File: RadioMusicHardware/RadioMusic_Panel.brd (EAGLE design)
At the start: 128.5 x 20 mm, 13 parts, among them X1 VERT_SD_CARD

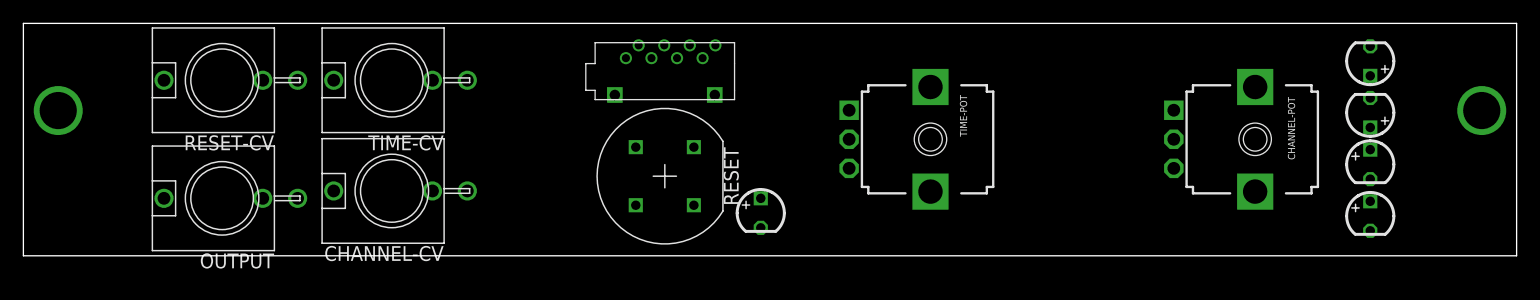
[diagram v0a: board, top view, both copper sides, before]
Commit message: Panel design
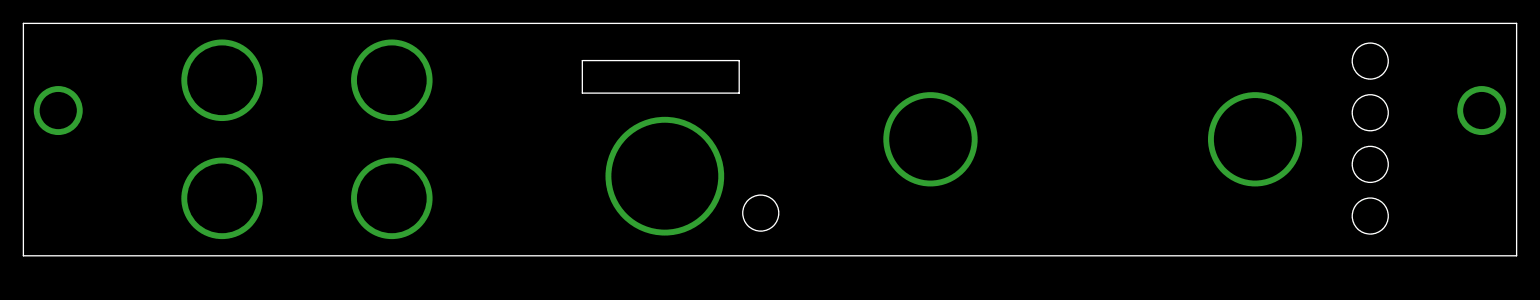
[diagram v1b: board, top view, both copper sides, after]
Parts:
- removed CHANNEL-CV, OUTPUT, RESET-CV, TIME-CV: (no value), thonkiconn:WQP-PJ301M-12_JACK
- removed CHANNEL-POT, TIME-POT: 50k, TomW:EVUF
- removed LED1, LED2, LED3, LED4, LED5: (no value), TomW:LED3MM
- removed RESET: D6_PUSH_SWITCH, TomW:D6_BUTTON_RND
- removed X1: VERT_SD_CARD, TomW:VERT_MICROSD
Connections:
- removed net +3.3V_F: TIME-POT.3
- removed net GND_F: CHANNEL-CV.P$3
- removed net LED3_F: LED3.A
- removed net LED4_F: LED4.A
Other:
- outline, holes or cut-outs redrawn
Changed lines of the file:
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@@
 <setting verticaltext="up"/>
 </settings>
-<grid distance="25" unitdist="mil" unit="mm" style="lines" multiple="1" display="yes" altdistance="8" altunitdist="mil" altunit="mil"/>
+<grid distance="25" unitdist="mil" unit="mm" style="lines" multiple="1" display="yes" altdistance="0.1" altunitdist="mm" altunit="mm"/>
 <layers>
 <layer number="1" name="Top" color="4" fill="1" visible="yes" active="yes"/>
@@
 <wire x1="128.5" y1="0" x2="128.5" y2="20" width="0.0254" layer="20"/>
 <wire x1="128.5" y1="20" x2="0" y2="20" width="0.0254" layer="20"/>
-<wire x1="130.75" y1="10" x2="-9.25" y2="10" width="0.1" layer="51"/>
-<wire x1="64.25" y1="-9.5" x2="64.25" y2="30.5" width="0.1" layer="51"/>
+<rectangle x1="48.1" y1="14" x2="61.6" y2="16.8" layer="46"/>
+<hole x="63.455" y="3.675" drill="3.1"/>
+<hole x="115.906" y="16.756" drill="3.1"/>
+<hole x="115.906" y="12.311" drill="3.1"/>
+<hole x="115.906" y="7.866" drill="3.1"/>
+<hole x="115.906" y="3.421" drill="3.1"/>
 </plain>
 <attributes>
@@
 </autorouter>
 <elements>
-<element name="CHANNEL-POT" library="TomW" package="EVUF" value="50k" x="106" y="10.025" smashed="yes" rot="R270">
-<attribute name="NAME" x="108.825" y="13.66" size="0.6096" layer="25" rot="R270"/>
-<attribute name="VALUE" x="101.58" y="11.985" size="0.6096" layer="27" rot="R270"/>
-</element>
-<element name="CHANNEL-CV" library="thonkiconn" package="WQP-PJ301M-12_JACK" value="" x="31.705" y="5.58" rot="R90"/>
-<element name="RESET-CV" library="thonkiconn" package="WQP-PJ301M-12_JACK" value="" x="17.1" y="15.105" rot="R90"/>
-<element name="OUTPUT" library="thonkiconn" package="WQP-PJ301M-12_JACK" value="" x="17.1" y="4.945" rot="R90"/>
-<element name="TIME-POT" library="TomW" package="EVUF" value="50k" x="78.06" y="10.025" smashed="yes" rot="R270">
-<attribute name="NAME" x="80.6" y="13.835" size="0.6096" layer="25" rot="R270"/>
-<attribute name="VALUE" x="74.25" y="13.835" size="0.6096" layer="27" rot="R270"/>
-</element>
-<element name="TIME-CV" library="thonkiconn" package="WQP-PJ301M-12_JACK" value="" x="31.705" y="15.105" rot="R90"/>
-<element name="RESET" library="TomW" package="D6_BUTTON_RND" value="D6_PUSH_SWITCH" x="55.2" y="6.85" rot="R180"/>
-<element name="LED1" library="TomW" package="LED3MM" value="" x="115.906" y="16.756" rot="R90"/>
-<element name="LED2" library="TomW" package="LED3MM" value="" x="115.906" y="12.311" rot="R90"/>
-<element name="LED3" library="TomW" package="LED3MM" value="" x="115.906" y="7.866" rot="R270"/>
-<element name="LED4" library="TomW" package="LED3MM" value="" x="115.906" y="3.421" rot="R270"/>
-<element name="X1" library="TomW" package="VERT_MICROSD" value="VERT_SD_CARD" x="55.2" y="17.01"/>
-<element name="LED5" library="TomW" package="LED3MM" value="" x="63.455" y="3.675" rot="R270"/>
 </elements>
 <signals>
 <signal name="VBAT">
 </signal>
-<signal name="LED4_F">
-<contactref element="LED4" pad="A"/>
-</signal>
-<signal name="LED3_F">
-<contactref element="LED3" pad="A"/>
-</signal>
-<signal name="+3.3V_F">
-<contactref element="TIME-POT" pad="3"/>
-</signal>
-<signal name="GND_F" class="2" airwireshidden="yes">
-<contactref element="CHANNEL-CV" pad="P$3"/>
-</signal>
-<signal name="N$1">
+<signal name="GND">
+<via x="17.1" y="15.105" extent="1-16" drill="6"/>
+<via x="31.705" y="15.105" extent="1-16" drill="6"/>
+<via x="17.1" y="4.945" extent="1-16" drill="6"/>
+<via x="31.705" y="4.945" extent="1-16" drill="6"/>
+<via x="55.2" y="6.85" extent="1-16" drill="9.2"/>
+<via x="78.06" y="10.025" extent="1-16" drill="7.1"/>
 <via x="3" y="12.5" extent="1-16" drill="3.2"/>
-</signal>
-<signal name="N$2">
+<via x="106" y="10.025" extent="1-16" drill="7.1"/>
 <via x="125.5" y="12.5" extent="1-16" drill="3.2"/>
+<wire x1="106" y1="10.025" x2="125.5" y2="12.5" width="0" layer="19" extent="1-1"/>
+<wire x1="78.06" y1="10.025" x2="106" y2="10.025" width="0" layer="19" extent="1-1"/>
+<wire x1="55.2" y1="6.85" x2="78.06" y2="10.025" width="0" layer="19" extent="1-1"/>
+<wire x1="31.705" y1="4.945" x2="55.2" y2="6.85" width="0" layer="19" extent="1-1"/>
+<wire x1="31.705" y1="15.105" x2="31.705" y2="4.945" width="0" layer="19" extent="1-1"/>
+<wire x1="17.1" y1="15.105" x2="31.705" y2="15.105" width="0" layer="19" extent="1-1"/>
+<wire x1="17.1" y1="4.945" x2="17.1" y2="15.105" width="0" layer="19" extent="1-1"/>
+<wire x1="3" y1="12.5" x2="17.1" y2="15.105" width="0" layer="19" extent="1-1"/>
 </signal>
 </signals>
